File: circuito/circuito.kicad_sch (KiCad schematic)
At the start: 7 parts, among them J1 Conn_01x04, J2 Screw_Terminal_01x03, SW1 Push_Button, SW2 Push_Button, U1 DS18B20

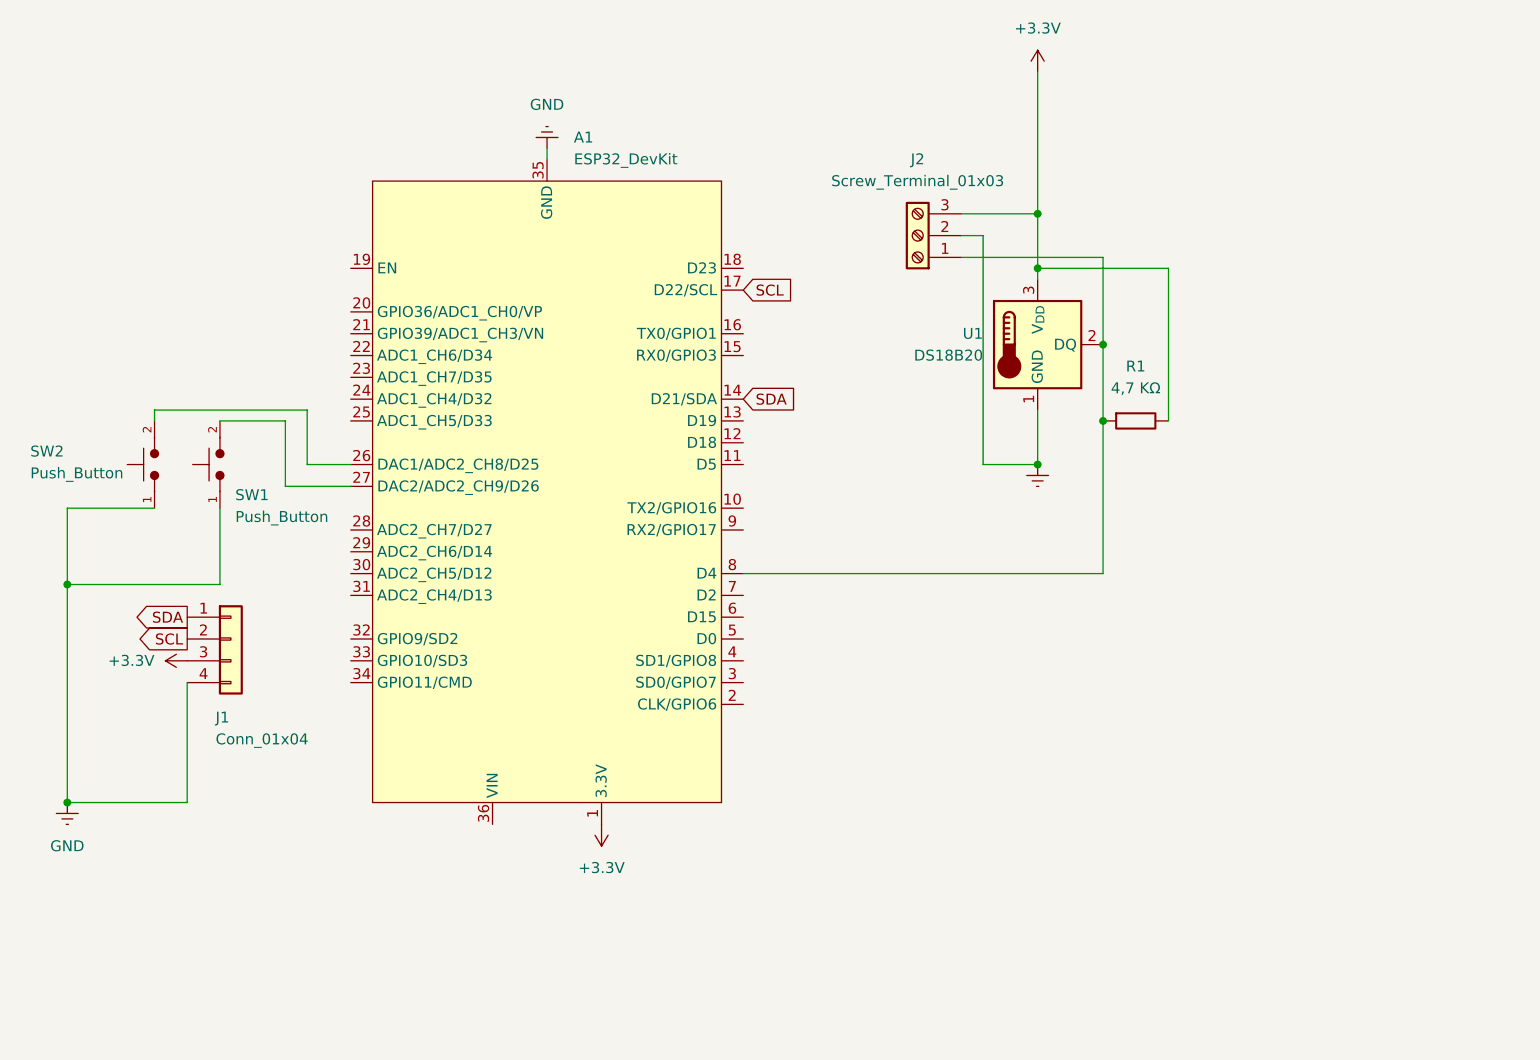
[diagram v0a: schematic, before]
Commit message: atualizando circuito
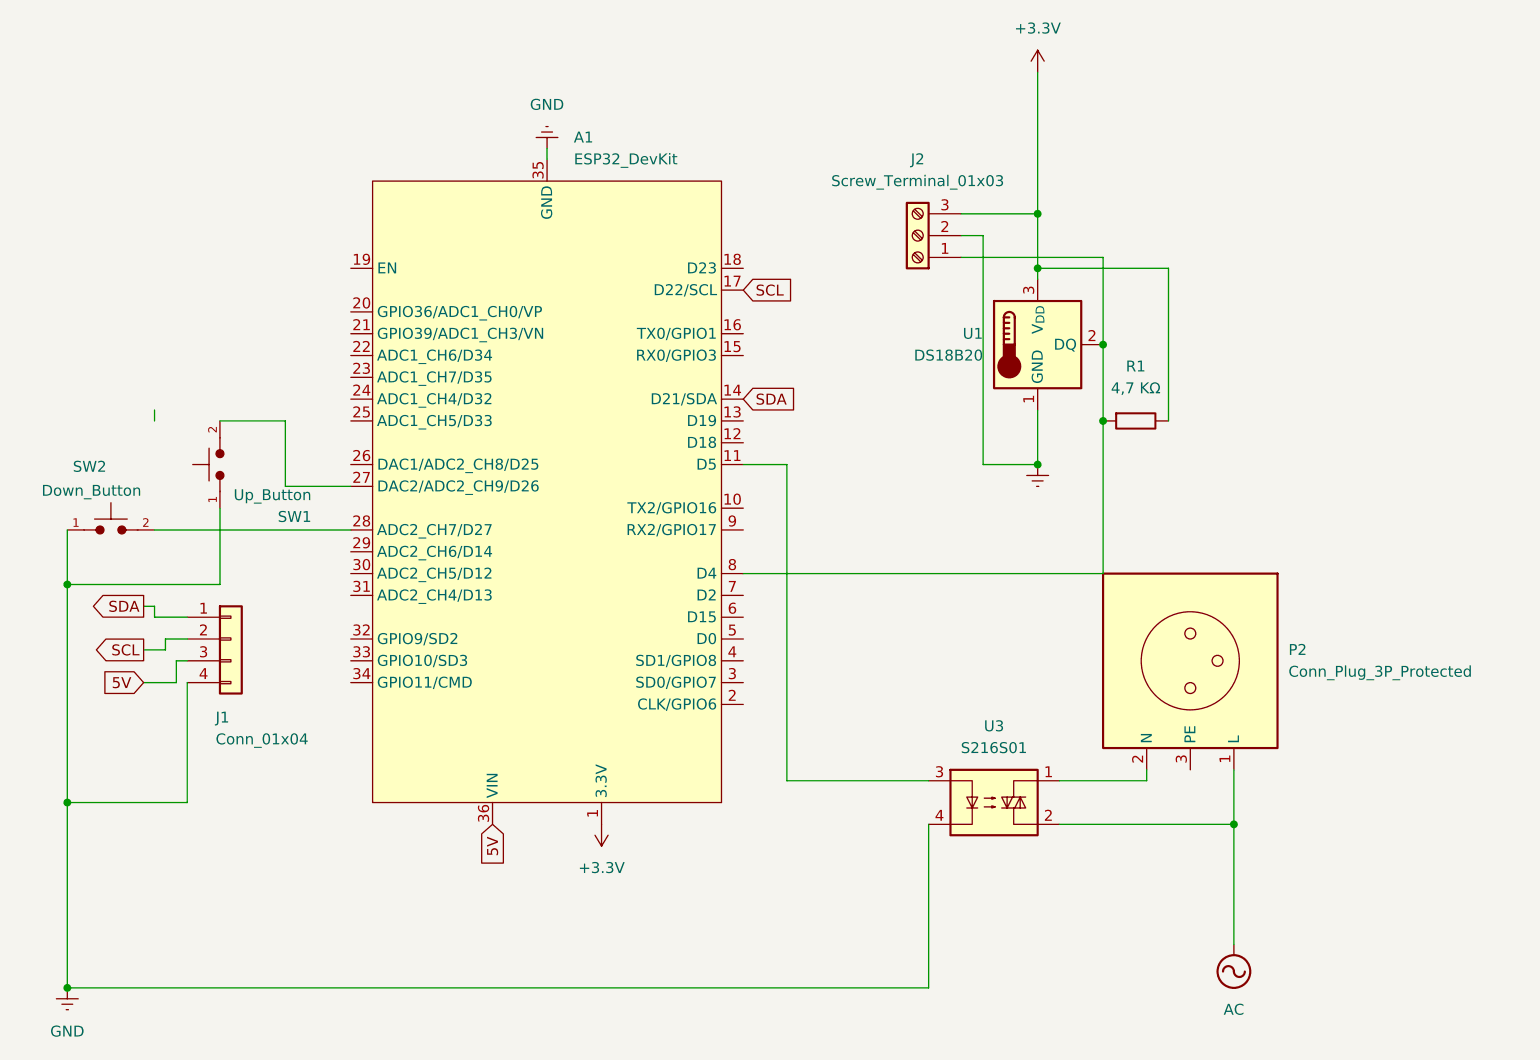
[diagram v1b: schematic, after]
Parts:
- added P2: Conn_Plug_3P_Protected, symbol Connector:Conn_Plug_3P_Protected
- added U3: S216S01, Package_SIP:SIP4_Sharp-SSR_P7.62mm_Straight, symbol Relay_SolidState:S216S01
- SW1: value Push_Button -> Up_Button
- SW2: value Push_Button -> Down_Button
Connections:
- net +3.3V: no longer J1.3 (Pin_3)
- net GND: now also U3.4
- net at SW2.2: now also A1.28 (ADC2_CH7/D27); no longer A1.26 (DAC1/ADC2_CH8/D25)
- net at A1.11 (D5): now also U3.3
- net 5V: now reaches A1.36 (VIN)
- net 5V: now also J1.3 (Pin_3)
- new net: P2.2 (N), U3.1
- new net AC: P2.1 (L), U3.2
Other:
- moved on the sheet: SW2
